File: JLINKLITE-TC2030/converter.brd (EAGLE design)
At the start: 30.5 x 72.9 mm, 13 parts

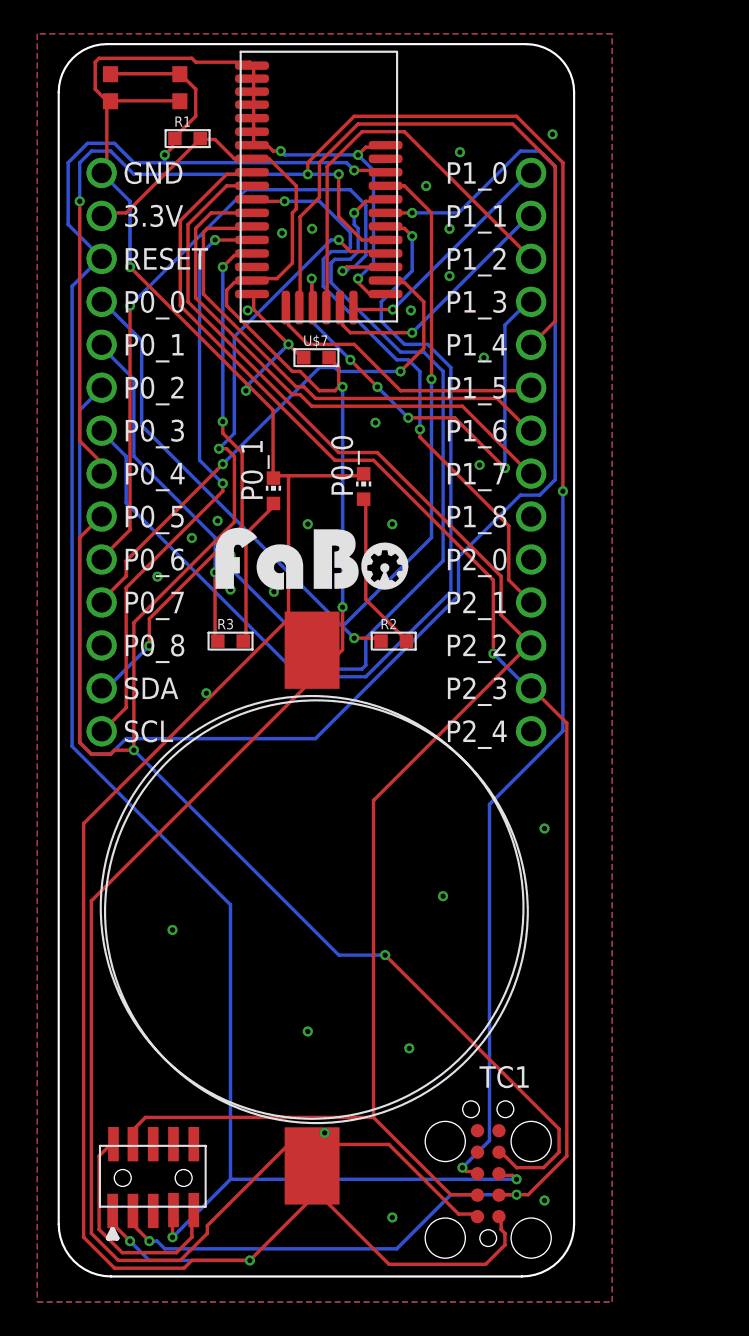
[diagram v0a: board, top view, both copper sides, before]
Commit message: Add update
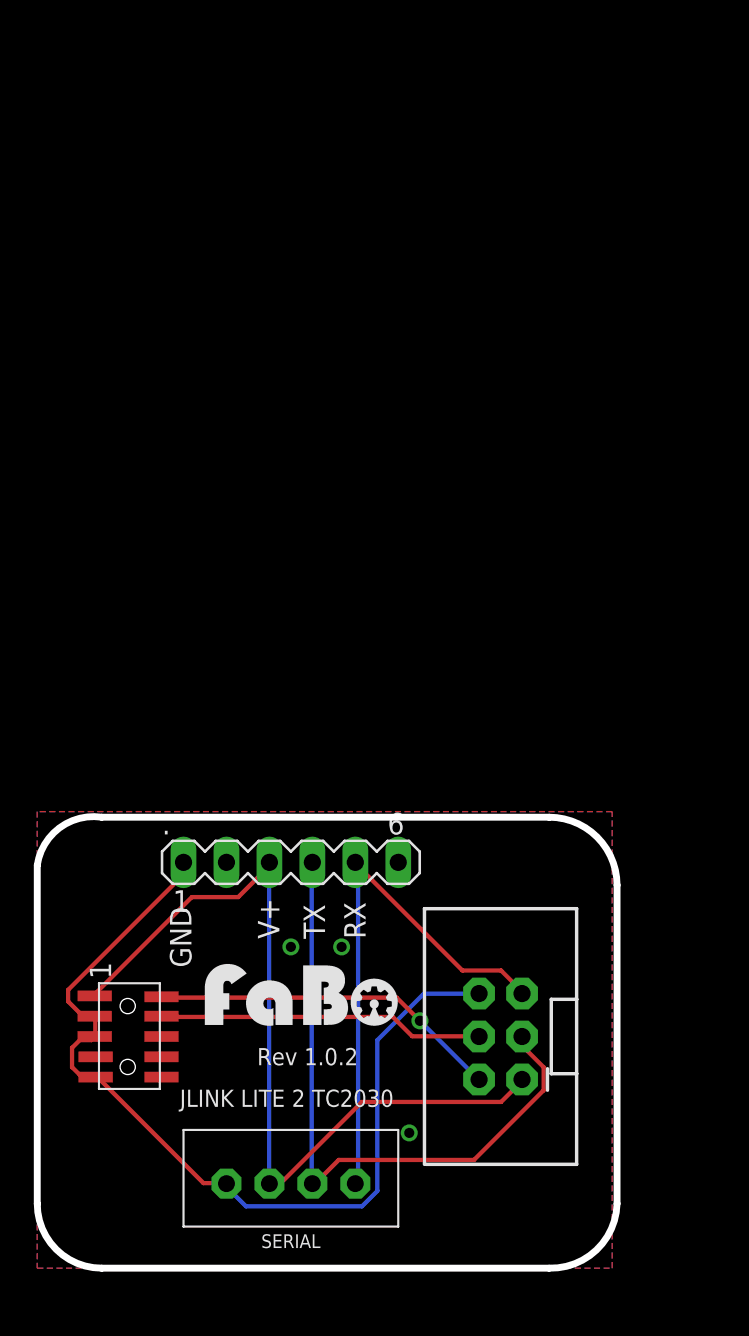
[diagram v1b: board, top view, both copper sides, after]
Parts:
- removed P0_0, P0_1: (no value), led:CHIP-LED0603
- removed R1: 10K, GClue-Resistors:0603
- removed R2, R3: 180, GClue-Resistors:0603
- removed TC1: TC2050-IDCB, TagConnect:TC2050-IDC
- removed U$2: BREAKOUT_BLE, gclue:BREAKOUT_BLE
- removed U$3: BLUEGIGA-BLE113, GClueBT:BLUEGIGA-BLE113
- removed U$4: SMTU2450-TOP, GClue-Supply:SMTU2450
- removed U$7: CAPACITOR0603, GClue-Capacitor:0603
- removed U$8: (no value), FaBo:LOGO_FABO_M
- added .: (no value), con-lstb:MA06-1
- added JP2: (no value), SparkFun-Connectors:2X3-SHROUDED
- added SERIAL: (no value), FaBo-Template:FABO_BRICK_SERIAL_CONNECTOR_I
- U$1: value PIN-HEADER-SMT(1.27MM)2X5 -> (none); device gclue:PIN-HEADER-SMT(1.27MM)2X5 -> FaBo:LOGO_FABO_M
- U$5: value SWICTH-4P(KMR2) -> PIN-HEADER-SMT(1.27MM)2X5; device gclue-test:SWITCH-4P(KMR2) -> GClue:PIN-HEADER-SMT(1.27MM)2X5
- moved U$5 56.9 mm to (5.35, 13.7), turned to 270 degrees
- moved U$1 12.6 mm to (15.6, 14.3)
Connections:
- removed net +3V3: U$1.2, U$1.9
- removed net DEBUG_CLOCK: TC1.4, U$1.4, U$2.P2_2, U$3.10
- removed net DEBUG_DATA: TC1.3, U$1.3, U$2.P2_3, U$3.9
- removed net N$12: U$2.P0_8
- removed net P0_0: R2.1, U$2.P0_0, U$3.33
- removed net P0_1: R3.1, U$2.P0_1, U$3.32
- removed net P0_2: U$2.P0_2, U$3.31
- removed net P0_3: U$2.P0_3, U$3.30
- removed net P0_4: TC1.6, U$2.P0_4, U$3.29
- removed net P0_5: TC1.7, U$2.P0_5, U$3.28
- removed net P0_6: U$2.P0_6, U$3.27
- removed net P0_7: U$2.P0_7, U$3.26
- removed net P1_0: U$2.P1_0, U$3.24
- removed net P1_1: U$2.P1_1, U$3.23
- removed net P1_2: U$2.P1_2, U$3.22
- removed net P1_3: U$2.P1_3, U$3.21
- removed net P1_4: U$2.P1_4, U$3.20
- removed net P1_5: U$2.P1_5, U$3.19
- removed net P1_6: U$2.P1_6, U$3.13
- removed net P1_7: U$2.P1_7, U$3.12
- removed net P1_8: U$2.P1_8
- removed net P1_9: U$2.P2_0
- removed net P2_0: U$2.P2_1, U$3.11
- removed net R1: P0_1.A, R3.2
- removed net R2: P0_0.A, R2.2
- removed net SCL: U$2.SCL, U$3.14
- removed net SDA: U$2.SDA, U$3.15
- new net RX: ..5, JP2.5, SERIAL.RX
- new net SWCLK: JP2.4, U$5.4
- new net SWDIO: JP2.2, U$5.2
- new net TX: ..4, JP2.3, SERIAL.TX
- net 3.3V: now also ..3, JP2.1, SERIAL.VCC, U$5.1; no longer R1.2, TC1.2, U$2.3.3V, U$3.17, U$3.8, U$4.P$_VCC, U$7.2
- net GND: now also ..1, JP2.6, SERIAL.GND, U$5.5, U$5.9; no longer P0_0.C, P0_1.C, TC1.1, U$1.1, U$2.GND, U$3.1, U$3.18, U$3.2, U$3.25, U$3.3, U$3.36, U$3.4, U$3.5, U$3.6, U$3.7, U$4.P$_GND, U$5.4, U$7.1
- net RESET: now also U$5.10; no longer R1.1, TC1.5, U$1.7, U$2.RESET, U$3.34, U$5.1, U$5.2
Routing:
- net P0_4: track 121.9 -> 0.00 mm, vias 5 -> 0
- net GND: track 176.3 -> 55.0 mm, vias 36 -> 3
- net RESET: track 120.8 -> 0.00 mm, vias 4 -> 0
- net DEBUG_DATA: track 102.1 -> 0.00 mm, vias 3 -> 0
- net P0_5: track 97.2 -> 0.00 mm, vias 4 -> 0
- net DEBUG_CLOCK: track 94.6 -> 0.00 mm
- net P0_2: track 88.4 -> 0.00 mm, vias 1 -> 0
- net 3.3V: track 123.0 -> 50.3 mm, vias 2 -> 0
- net P0_1: track 67.4 -> 0.00 mm, vias 2 -> 0
- net P0_0: track 57.8 -> 0.00 mm, vias 2 -> 0
- net P0_3: track 56.5 -> 0.00 mm, vias 1 -> 0
- net P0_6: track 40.2 -> 0.00 mm, vias 2 -> 0
- net TX: track 0.00 -> 38.7 mm
- net P1_4: track 36.1 -> 0.00 mm
- net P2_0: track 35.2 -> 0.00 mm, vias 2 -> 0
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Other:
- board size 30.5 x 72.9 mm -> 34.3 x 26.7 mm
- board text added: "GND"
- board text added: "JLINK LITE 2 TC2030"
- board text added: "RX"
- board text added: "Rev 1.0.2"
- board text added: "TX"
- board text added: "V+"
- board text removed: "Rev.Beat20150902"

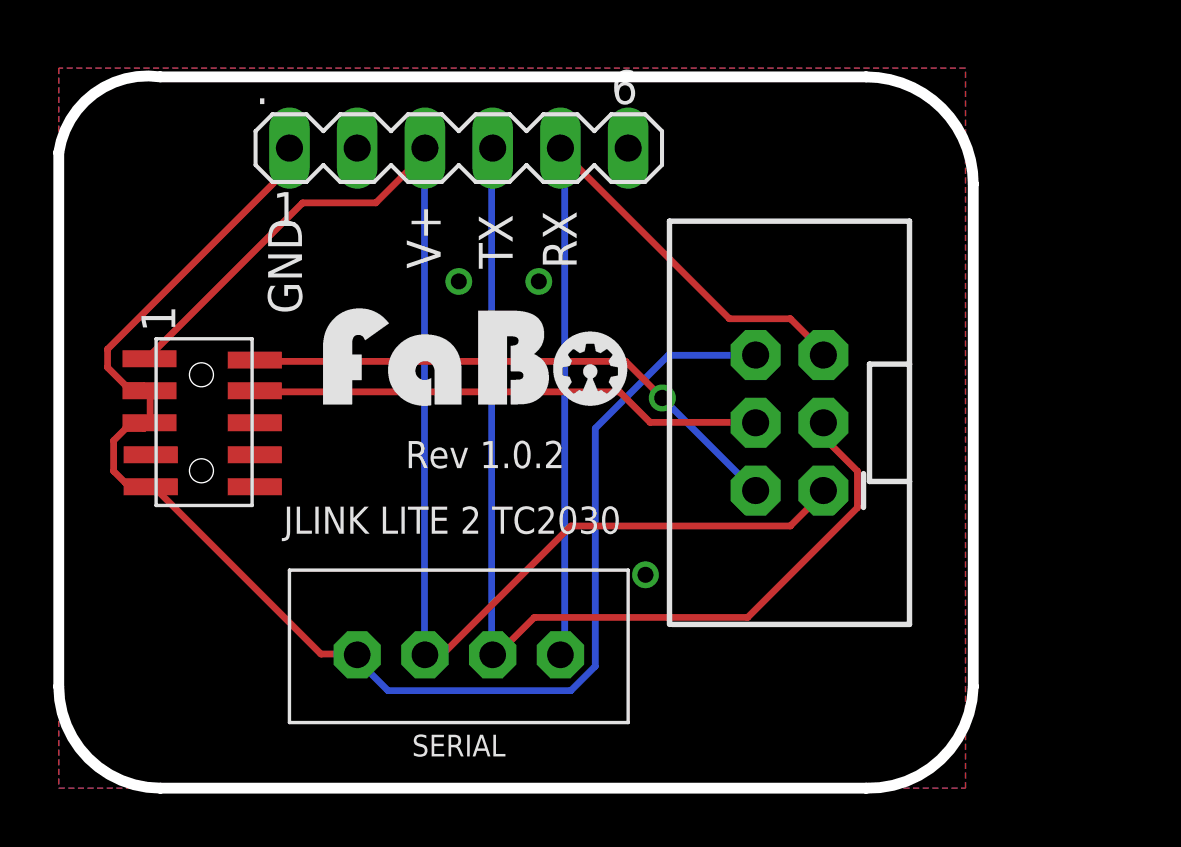
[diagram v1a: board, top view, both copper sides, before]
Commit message: Update new meme.
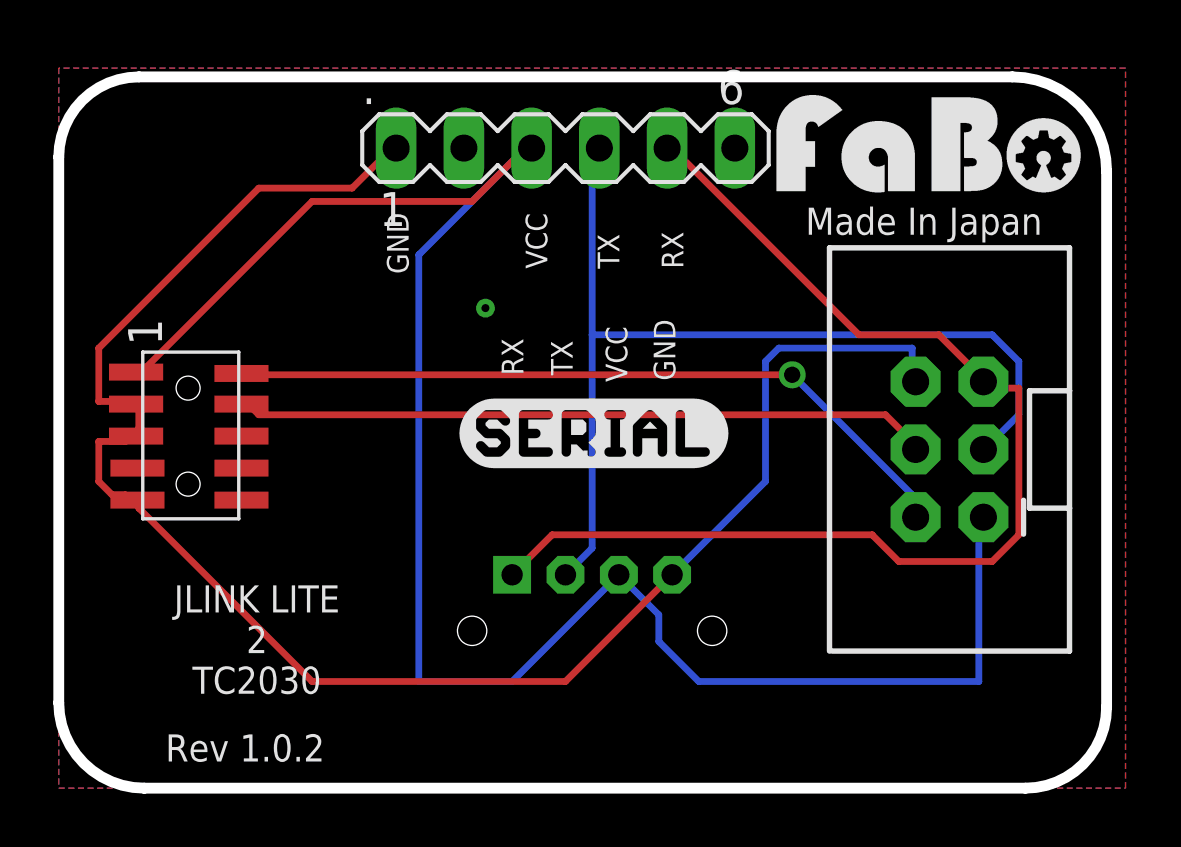
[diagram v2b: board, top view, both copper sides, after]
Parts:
- removed SERIAL: (no value), FaBo-Template:FABO_BRICK_SERIAL_CONNECTOR_I
- added ..: (no value), FaBo-Template:FABO_BRICK_SERIAL_S04B-PASK-2
- added U$2: (no value), FaBo-etc:LOGO_SILK_SERIAL2
- moved U$1 18.8 mm to (32.6, 22.3)
- moved JP2 6.08 mm to (33.4, 12.7)
- moved . 4.00 mm to (19.0, 24.0)
- moved U$5 0.71 mm to (4.85, 13.2)
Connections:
- net 3.3V: now also ...VCC; no longer SERIAL.VCC
- net GND: now also ...GND; no longer SERIAL.GND
- net RX: now also ...RX; no longer SERIAL.RX
- net TX: now also ...TX; no longer SERIAL.TX
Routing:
- net 3.3V: track 50.3 -> 71.4 mm
- net RX: track 32.3 -> 42.9 mm
- net GND: track 55.0 -> 64.9 mm, vias 3 -> 1
- net SWDIO: track 20.8 -> 27.9 mm
- net SWCLK: track 19.3 -> 26.1 mm
- net TX: track 38.7 -> 37.0 mm
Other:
- board size 34.3 x 26.7 mm -> 39.3 x 26.7 mm
- board text added: "Made In Japan"
- board text added: "VCC"
- board text removed: "V+"
